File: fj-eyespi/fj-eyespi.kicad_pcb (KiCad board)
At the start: 2 copper layers, 45.6 x 30.7 mm, 2 parts, among them J1 Conn_01x18_Socket, J2 FruitJam-2x16

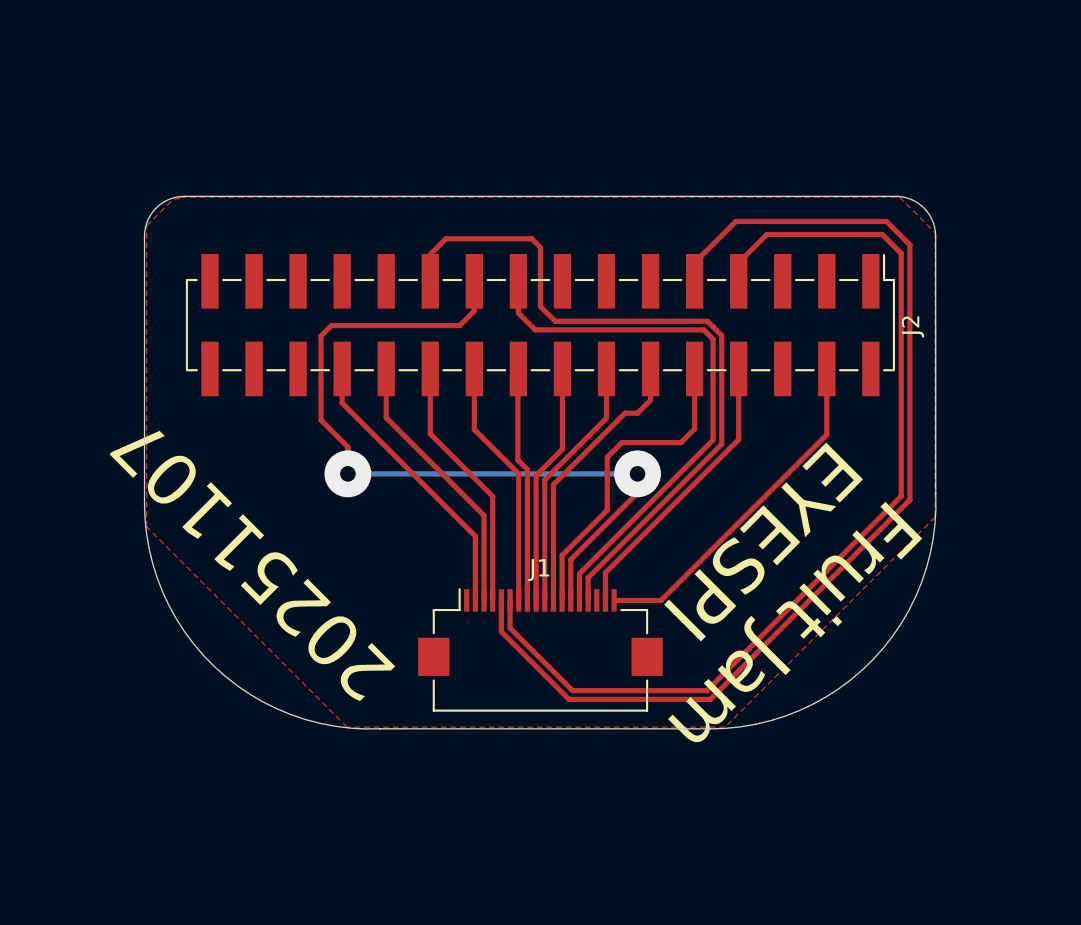
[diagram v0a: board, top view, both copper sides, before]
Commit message: sync
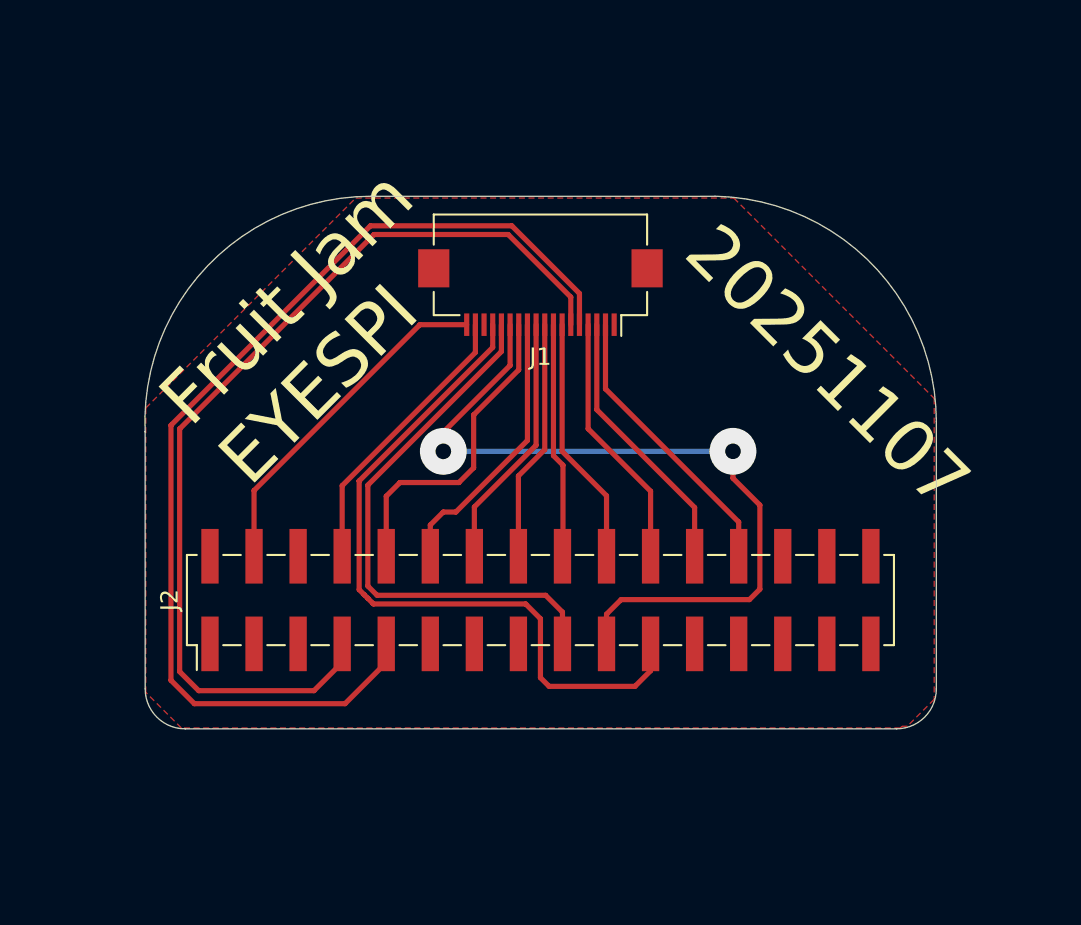
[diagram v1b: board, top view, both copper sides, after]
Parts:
- moved J1 19.6 mm to (155.9, 75.5), turned to 180 degrees
- moved J2 15.9 mm to (155.9, 93.3), turned to 90 degrees
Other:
- outline, holes or cut-outs redrawn
